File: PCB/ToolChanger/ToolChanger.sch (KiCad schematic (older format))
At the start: 23 parts, among them J1 Conn_01x26_Male, J2 Con_Motor, J3 Conn_01x06, J4 Conn_01x02, U1 STM32L-Discovery, U2 PC817, U3 PC817, U4 PC817, U5 PC817

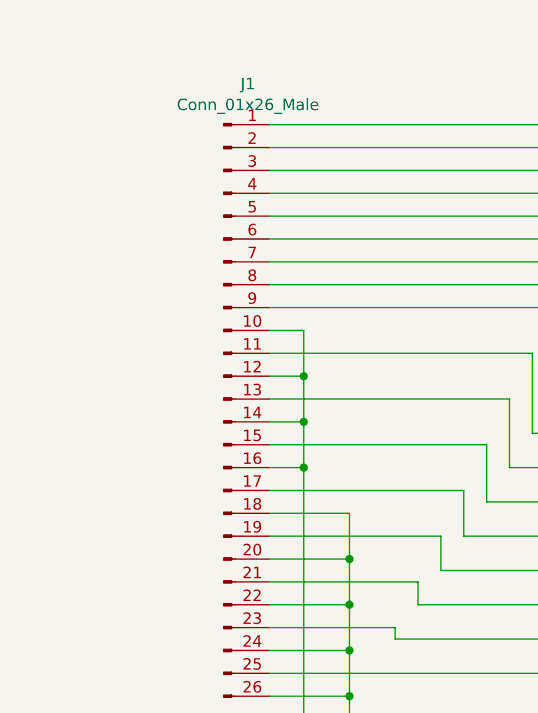
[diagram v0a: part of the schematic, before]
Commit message: Initial commit. Toolchange working
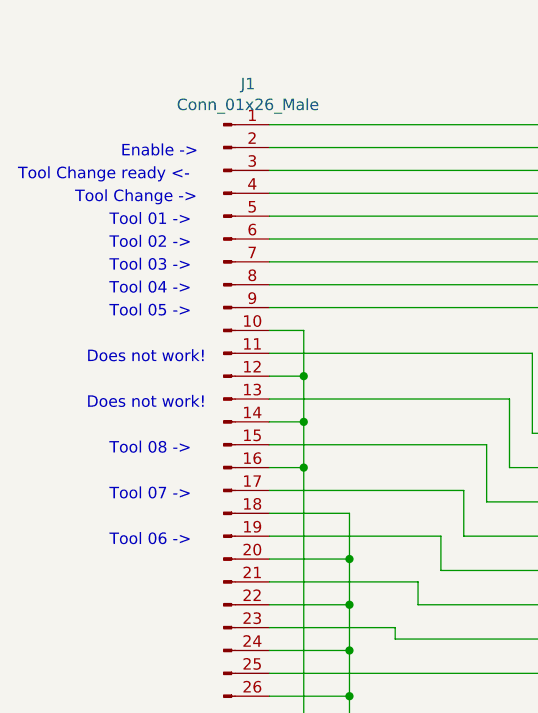
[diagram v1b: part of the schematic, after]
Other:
- note added: "Does not work!"
- note added: "Enable ->"
- note added: "Tool 01 ->"
- note added: "Tool 02 ->"
- note added: "Tool 03 ->"
- note added: "Tool 04 ->"
- note added: "Tool 05 ->"
- note added: "Tool 06 ->"
- note added: "Tool 07 ->"
- note added: "Tool 08 ->"
- note added: "Tool Change ->"
- note added: "Tool Change ready <-"
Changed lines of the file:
@@
 EESchema Schematic File Version 4
+LIBS:ToolChanger-cache
 EELAYER 26 0
 EELAYER END
@@
 	1    0    0    -1
 $EndComp
+Text Notes 1000 1550 0    50   ~ 0
+Enable ->
+Text Notes 550  1650 0    50   ~ 0
+Tool Change ready <-
+Text Notes 800  1750 0    50   ~ 0
+Tool Change ->
+Text Notes 950  1850 0    50   ~ 0
+Tool 01 ->
+Text Notes 950  1950 0    50   ~ 0
+Tool 02 ->
+Text Notes 950  2050 0    50   ~ 0
+Tool 03 ->
+Text Notes 950  2150 0    50   ~ 0
+Tool 04 ->
+Text Notes 950  2250 0    50   ~ 0
+Tool 05 ->
+Text Notes 950  3250 0    50   ~ 0
+Tool 06 ->
+Text Notes 950  3050 0    50   ~ 0
+Tool 07 ->
+Text Notes 950  2850 0    50   ~ 0
+Tool 08 ->
+Text Notes 850  2450 0    50   ~ 0
+Does not work!
+Text Notes 850  2650 0    50   ~ 0
+Does not work!
 $EndSCHEMATC
